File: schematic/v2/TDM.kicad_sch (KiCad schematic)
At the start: 17 parts, among them J18 LCD_display, U5 24LC256-I_SN, U6 BME280, U8 24LC256-I_SN, U9 NUCLEO-F446RE

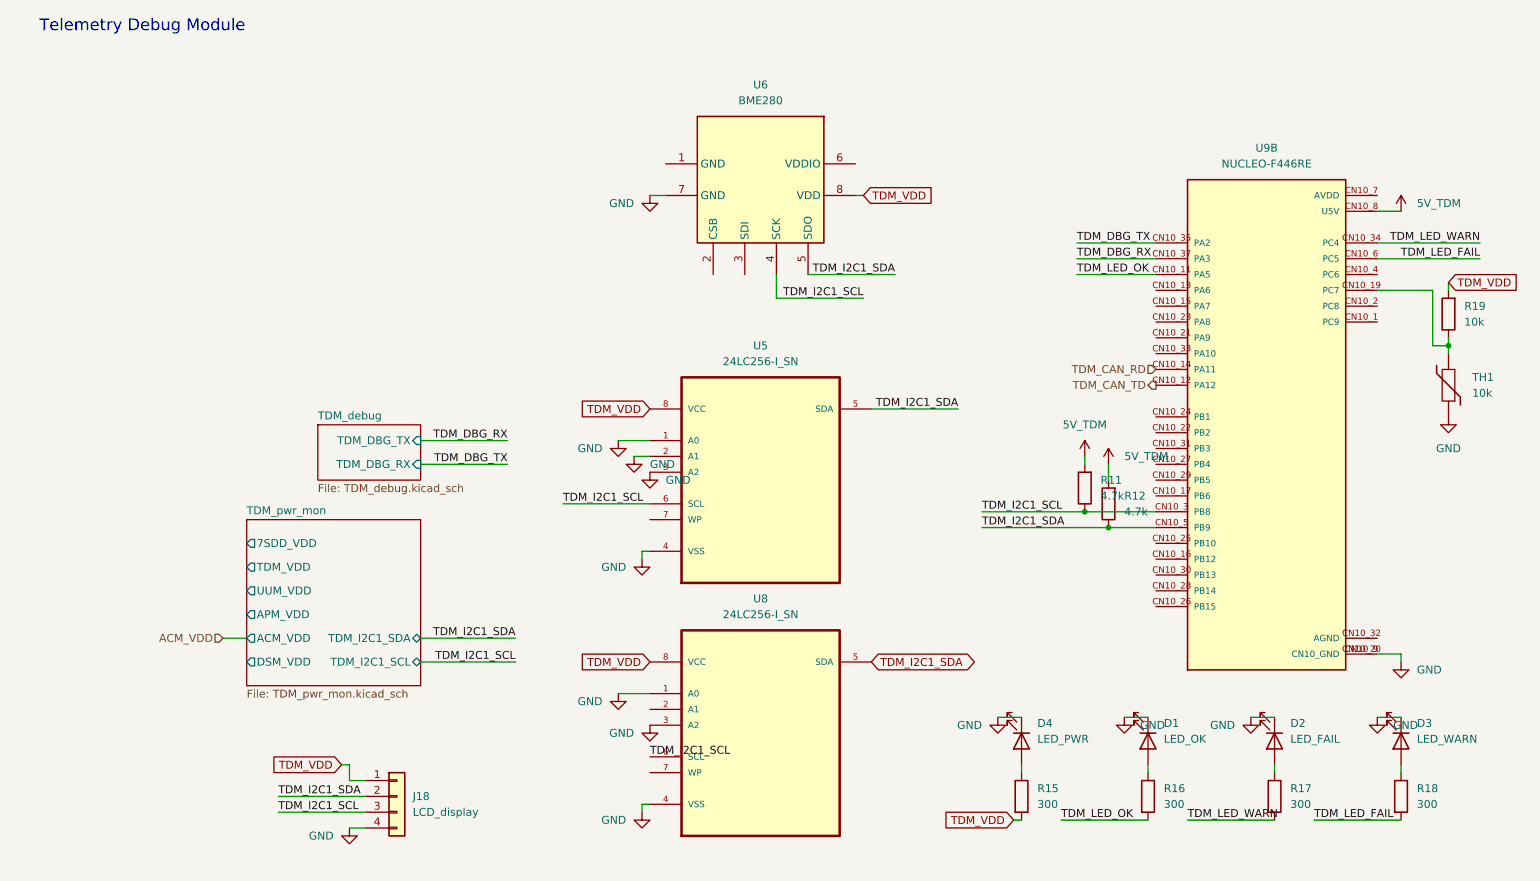
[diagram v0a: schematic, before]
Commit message: no errors in the ERC!
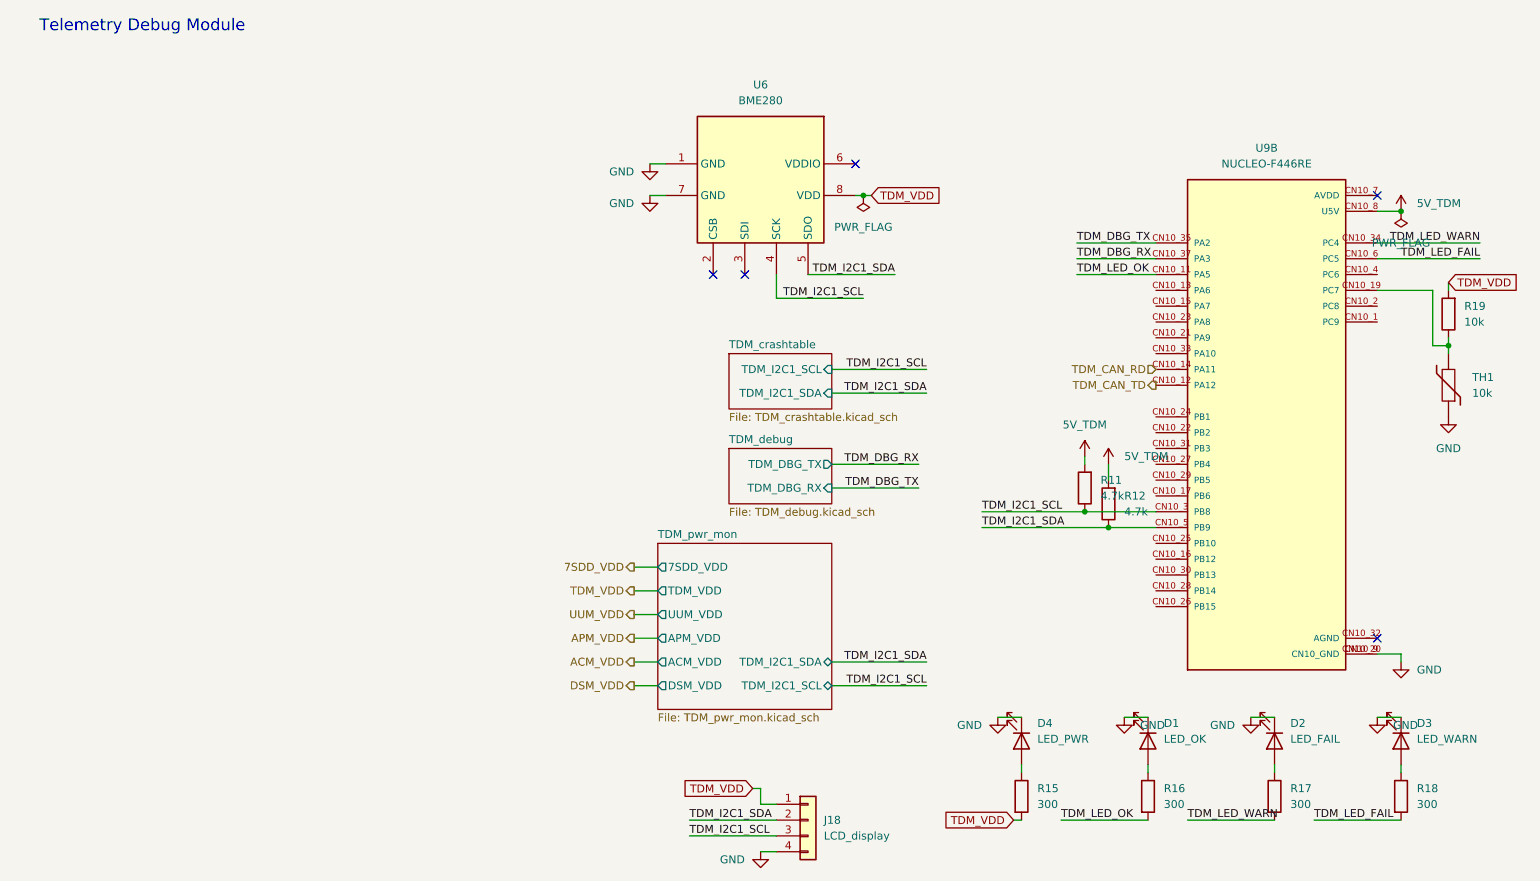
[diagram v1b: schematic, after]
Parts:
- removed U5, U8: 24LC256-I_SN, 24LC256-I_SN:SOIC127P600X175-8N, symbol 24LC256-I_SN:24LC256-I_SN
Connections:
- net GND: now also U6.1 (GND)
- no-connect marks 0 -> 5
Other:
- added sheet TDM_crashtable (TDM_crashtable.kicad_sch)
- moved on the sheet: J18
